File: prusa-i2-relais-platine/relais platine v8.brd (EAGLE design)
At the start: 160 x 100 mm, 8 parts, among them X1 IN-12V, X2 NOZ-FAN, X3 LIGHT, X4 BLK-FAN

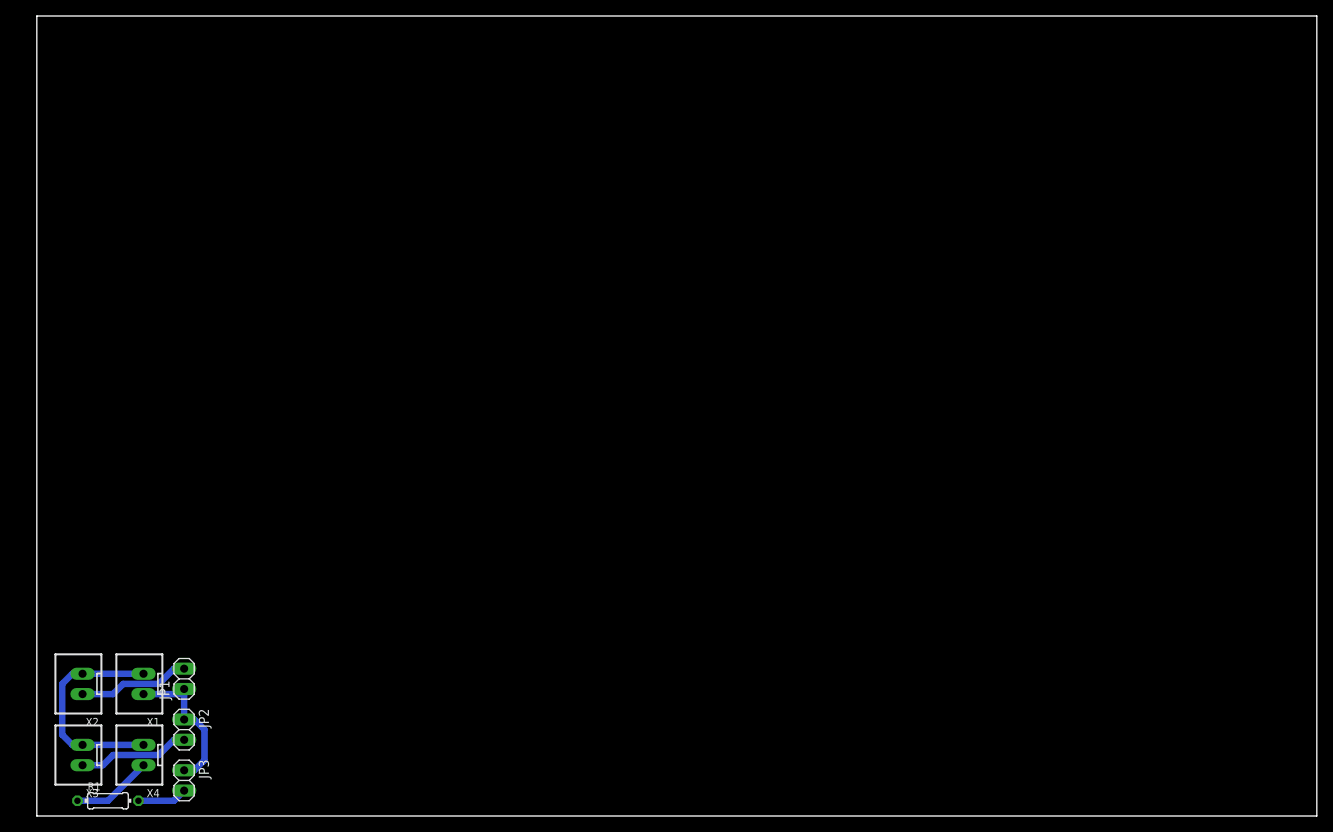
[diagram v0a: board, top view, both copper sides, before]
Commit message: new projects
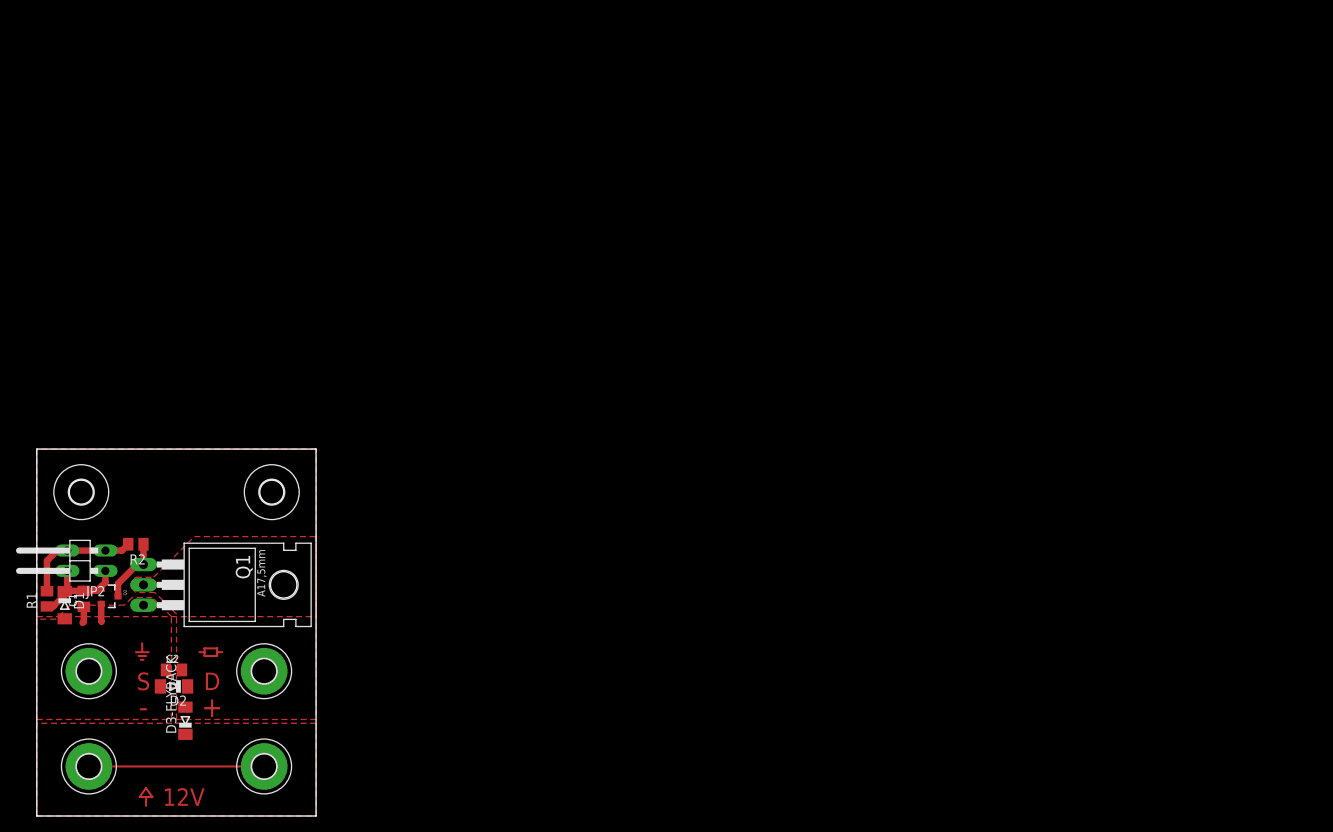
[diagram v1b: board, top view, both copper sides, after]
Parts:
- removed JP3: (no value), pinhead:1X02
- removed X1: IN-12V, Rembrandt Electronics - JST XH Connectors v1-0:JST-XH-02-PACKAGE-LONG-PAD
- removed X2: NOZ-FAN, Rembrandt Electronics - JST XH Connectors v1-0:JST-XH-02-PACKAGE-LONG-PAD
- removed X3: LIGHT, Rembrandt Electronics - JST XH Connectors v1-0:JST-XH-02-PACKAGE-LONG-PAD
- removed X4: BLK-FAN, Rembrandt Electronics - JST XH Connectors v1-0:JST-XH-02-PACKAGE-LONG-PAD
- added C1, C2: 100n, rcl:C0805K
- added D1, D2, D3-FLYBACK: (no value), diode:MINIMELF
- added H1, H2, H3, H4: M3, holes:3,0-PAD
- added Q1: IRF1404, transistor-fet:TO220
- added Q2: BS170, SparkFun-DiscreteSemi:SOT23-3
- added R2: 100k, rcl:M0805
- added U$1, U$2: (no value), holes:3,0
- JP2: device pinhead:1X02 -> pinhead:1X02/90
- R1: value (none) -> 100k; device rcl:0204/7 -> rcl:M0805
- moved R1 26.4 mm to (1.27, 27.1), turned to 90 degrees
- moved JP2 25.1 mm to (4.76, 31.9), turned to 90 degrees
- moved JP1 20.8 mm to (3.81, 31.9), flipped to the bottom
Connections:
- removed net N$1: JP1.2, X2.1
- removed net N$2: JP2.2, X3.1
- removed net N$3: R1.1, X4.1
- removed net N$4: JP3.2, R1.2
- new net !HEAT: C1.2, D1.C, JP1.1, JP2.1, Q2.1, R1.1
- new net HEAT: Q1.1, Q2.3, R2.1
- new net HIGH: C2.2, D2.C, D3-FLYBACK.A, H1.B3,0, Q1.2
- net +12V: now also D3-FLYBACK.C, H3.B3,0, H4.B3,0, JP1.2, JP2.2, R1.2, R2.2; no longer JP1.1, JP2.1, JP3.1, X1.1
- net GND: now also C1.1, C2.1, D1.A, D2.A, H2.B3,0, Q1.3, Q2.2; no longer X1.2, X2.2, X3.2, X4.2
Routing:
- net GND: track 27.7 -> 4.33 mm
- net +12V: track 18.8 -> 36.7 mm
- net N$1: track 14.0 -> 0.00 mm
- net !HEAT: track 0.00 -> 13.0 mm
- net N$2: track 14.0 -> 1.11 mm
- net N$3: track 10.1 -> 1.11 mm
- net HEAT: track 0.00 -> 8.29 mm
- net N$7: track 0.00 -> 6.35 mm
- net N$4: track 6.24 -> 1.59 mm
- net N$8: track 0.00 -> 4.32 mm
- net N$5: track 0.00 -> 0.95 mm
- added copper zone on layer 1, net +12V
- added copper zone on layer 1, net GND
- added copper zone on layer 1, net HIGH
- added copper zone on layer 1, net N$1
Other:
- board size 160 x 100 mm -> 34.9 x 45.9 mm
- board text added: "+"
- board text added: "-"
- board text added: "12V"
- board text added: "D"
- board text added: "S"
